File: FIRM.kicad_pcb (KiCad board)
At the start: 4 copper layers, 40.5 x 40.5 mm, 98 parts, among them J2 DM3CS-SF, Q2 IRLML6402, U1 STM32F405RGTx, U2 MIC5219-3.3YM5, U6 A-USBC-20F0-EA-GSR05, U7 W25Q128JVS, X2 32.768khz, Y1 12 MHz

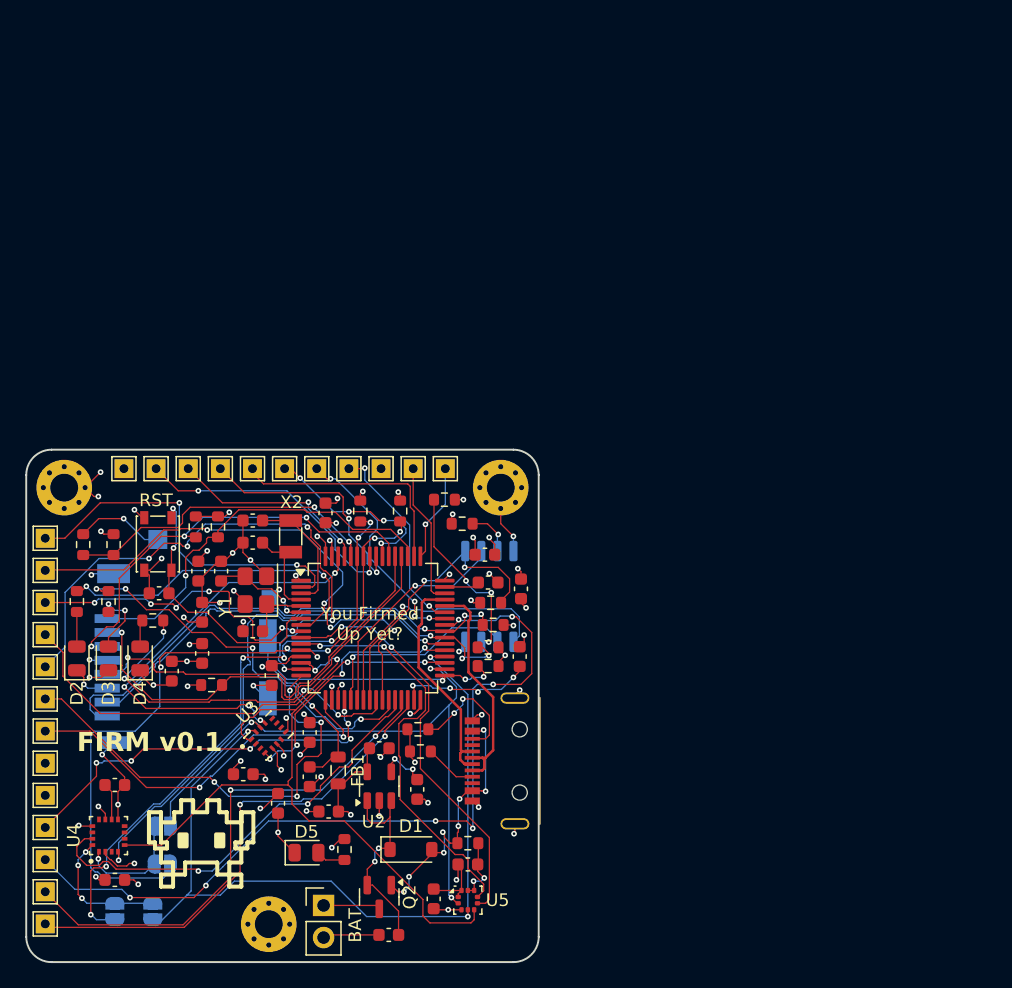
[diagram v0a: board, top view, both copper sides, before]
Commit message: sub 600
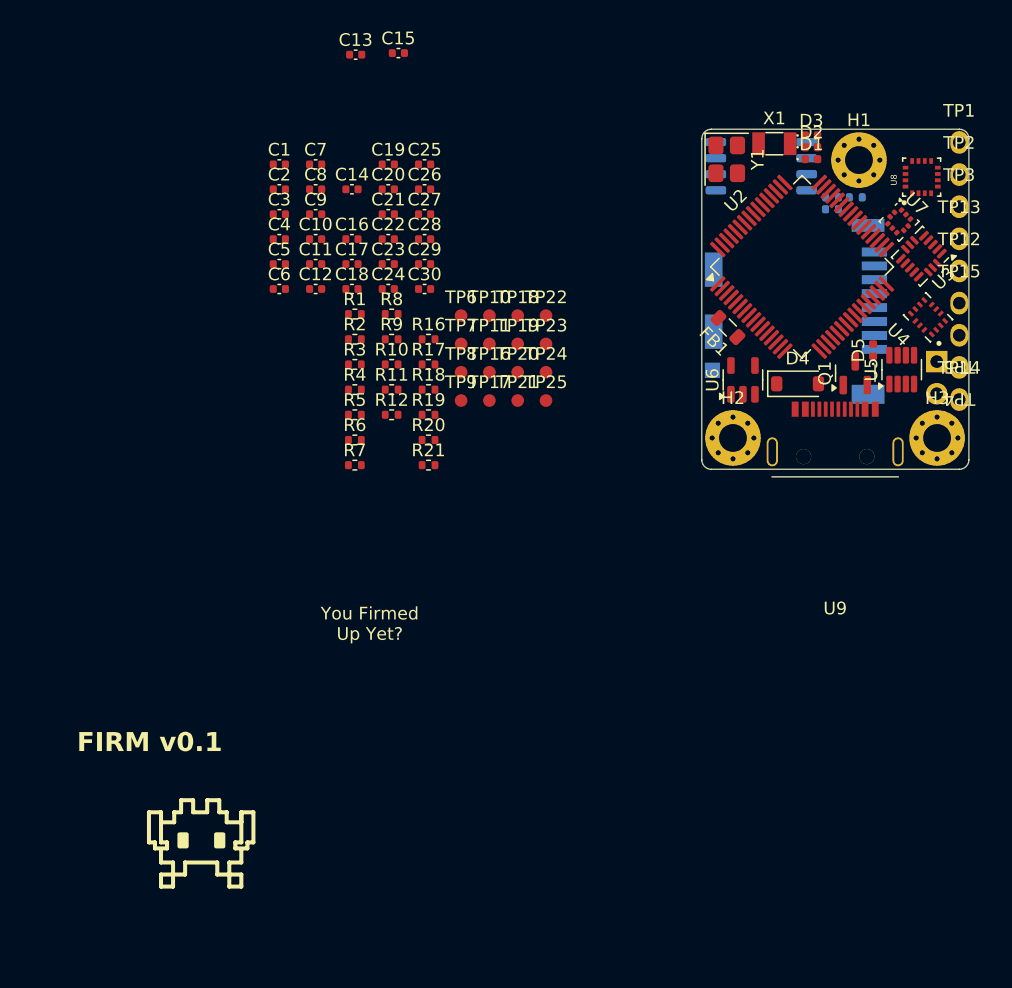
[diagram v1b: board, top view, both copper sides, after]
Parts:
- removed 3.3V: 3.3V Test Point, TestPoint:TestPoint_THTPad_1.5x1.5mm_Drill0.7mm
- removed A0: PA0 Test Point, TestPoint:TestPoint_THTPad_1.5x1.5mm_Drill0.7mm
- removed A1: PA1 Test Point, TestPoint:TestPoint_THTPad_1.5x1.5mm_Drill0.7mm
- removed A10: PA10 Test Point, TestPoint:TestPoint_THTPad_1.5x1.5mm_Drill0.7mm
- removed A15: PA15 Test Point, TestPoint:TestPoint_THTPad_1.5x1.5mm_Drill0.7mm
- removed A2: PA2 Test Point, TestPoint:TestPoint_THTPad_1.5x1.5mm_Drill0.7mm
- removed A3: PA3 Test Point, TestPoint:TestPoint_THTPad_1.5x1.5mm_Drill0.7mm
- removed A4: PA4 Test Point, TestPoint:TestPoint_THTPad_1.5x1.5mm_Drill0.7mm
- removed A8: PA8 Test Point, TestPoint:TestPoint_THTPad_1.5x1.5mm_Drill0.7mm
- removed A9: PA9 Test Point, TestPoint:TestPoint_THTPad_1.5x1.5mm_Drill0.7mm
- removed B10: PB10 Test Point, TestPoint:TestPoint_THTPad_1.5x1.5mm_Drill0.7mm
- removed B11: PB11 Test Point, TestPoint:TestPoint_THTPad_1.5x1.5mm_Drill0.7mm
- removed B3: PB3 Test Point, TestPoint:TestPoint_THTPad_1.5x1.5mm_Drill0.7mm
- removed B4: PB4 Test Point, TestPoint:TestPoint_THTPad_1.5x1.5mm_Drill0.7mm
- removed B5: PB5 Test Point, TestPoint:TestPoint_THTPad_1.5x1.5mm_Drill0.7mm
- removed B8: PB8 Test Point, TestPoint:TestPoint_THTPad_1.5x1.5mm_Drill0.7mm
- removed BAT: Conn_01x02_Pin, Connector_PinHeader_2.54mm:PinHeader_1x02_P2.54mm_Vertical
- removed BOOT0: BOOT0 Pad, TestPoint:TestPoint_Pad_1.5x1.5mm
- removed C0: PC0 Test Point, TestPoint:TestPoint_THTPad_1.5x1.5mm_Drill0.7mm
- removed the C13 at (101.5, 107.0)
- removed the C13 at (117.9, 114.3)
- removed GND (x2): GND Test Point, TestPoint:TestPoint_THTPad_1.5x1.5mm_Drill0.7mm
- removed GND: GND Through-Hole, TestPoint:TestPoint_THTPad_1.5x1.5mm_Drill0.7mm
- removed MOSI: SPI_SDI, Jumper:SolderJumper-2_P1.3mm_Open_RoundedPad1.0x1.5mm
- removed Q2: IRLML6402, Package_TO_SOT_SMD:SOT-23
- removed R22: 5.1k, Resistor_SMD:R_0603_1608Metric
- removed RST: PTS815, Button_Switch_SMD:SW_SPST_PTS810
- removed SCK: SPI_SCK, Jumper:SolderJumper-2_P1.3mm_Open_RoundedPad1.0x1.5mm
- removed SCL: I2C_SCL, Jumper:SolderJumper-2_P1.3mm_Open_RoundedPad1.0x1.5mm
- removed SDA: I2C_SDA, Jumper:SolderJumper-2_P1.3mm_Open_RoundedPad1.0x1.5mm
- removed SWCLK: SWCLK Through-Hole, TestPoint:TestPoint_THTPad_1.5x1.5mm_Drill0.7mm
- removed SWDIO: SWDIO Through-Hole, TestPoint:TestPoint_THTPad_1.5x1.5mm_Drill0.7mm
- removed TP30: PC1 Test Point, TestPoint:TestPoint_THTPad_1.5x1.5mm_Drill0.7mm
- removed X2: 32.768khz, Crystal:Crystal_SMD_3215-2Pin_3.2x1.5mm
- added C13: 100n, Capacitor_SMD:C_0402_1005Metric, F.Cu at (126.0, 68.8)
- added C28: 10u, Capacitor_SMD:C_0402_1005Metric, F.Cu at (131.5, 83.4)
- added C29: 1u, Capacitor_SMD:C_0402_1005Metric, F.Cu at (131.5, 85.3)
- added C30: 10u, Capacitor_SMD:C_0402_1005Metric, F.Cu at (131.5, 87.3)
- added J1: DM3CS-SF, connectors:HRS_DM3CS-SF, B.Cu at (160.7, 88.9)
- added Q1: IRLML6402, Package_TO_SOT_SMD:SOT-23, F.Cu at (165.5, 94.0)
- added R16: 100k, Resistor_SMD:R_0402_1005Metric, F.Cu at (131.8, 91.3)
- added R17: 0.01R, Resistor_SMD:R_0402_1005Metric, F.Cu at (131.8, 93.3)
- added TP1: PA0 Test Point, connectors:Testpoint_1.5x1.5mm_1.0mm, F.Cu at (173.7, 75.7)
- added TP10: I2C1_SCL Test Point, connectors:smd_test_pads_1mm, F.Cu at (136.6, 89.4)
- added TP11: I2C1_SDA Test Point, connectors:smd_test_pads_1mm, F.Cu at (136.6, 91.6)
- added TP12: SWDIO Through-Hole, connectors:Testpoint_1.5x1.5mm_1.0mm, F.Cu at (173.7, 85.9)
- added TP13: SWCLK Through-Hole, connectors:Testpoint_1.5x1.5mm_1.0mm, F.Cu at (173.7, 83.3)
- added TP14: 3.3V Test Point, connectors:Testpoint_1.5x1.5mm_1.0mm, F.Cu at (173.7, 96.0)
- added TP15: GND Test Point, connectors:Testpoint_1.5x1.5mm_1.0mm, F.Cu at (173.7, 88.4)
- added TP16: IMU_CS Test Point, connectors:smd_test_pads_1mm, F.Cu at (136.6, 93.9)
- added TP17: BMP_CS Test Point, connectors:smd_test_pads_1mm, F.Cu at (136.6, 96.1)
- added TP18: MAG_CS Test Point, connectors:smd_test_pads_1mm, F.Cu at (138.8, 89.4)
- added TP19: HIG_CS Test Point, connectors:smd_test_pads_1mm, F.Cu at (138.8, 91.6)
- added TP2: PA1 Test Point, connectors:Testpoint_1.5x1.5mm_1.0mm, F.Cu at (173.7, 78.3)
- added TP20: IMU_INT Test Point, connectors:smd_test_pads_1mm, F.Cu at (138.8, 93.9)
- added TP21: BMP_INT Test Point, connectors:smd_test_pads_1mm, F.Cu at (138.8, 96.1)
- added TP22: MAG_INT Test Point, connectors:smd_test_pads_1mm, F.Cu at (141.1, 89.4)
- added TP23: HIG_INT Test Point, connectors:smd_test_pads_1mm, F.Cu at (141.1, 91.6)
- added TP24: NRST Pad, connectors:smd_test_pads_1mm, F.Cu at (141.1, 93.9)
- added TP25: BOOT0 Pad, connectors:smd_test_pads_1mm, F.Cu at (141.1, 96.1)
- added TP3: PA2 Test Point, connectors:Testpoint_1.5x1.5mm_1.0mm, F.Cu at (173.7, 80.8)
- added TP4: PA9 Test Point, connectors:Testpoint_1.5x1.5mm_1.0mm, F.Cu at (173.7, 93.5)
- added TP5: PA10 Test Point, connectors:Testpoint_1.5x1.5mm_1.0mm, F.Cu at (173.7, 91.0)
- added TP6: PA4 Test Point, connectors:smd_test_pads_1mm, F.Cu at (134.4, 89.4)
- added TP7: MOSI2 Test Point, connectors:smd_test_pads_1mm, F.Cu at (134.4, 91.6)
- added TP8: MISO2 Test Point, connectors:smd_test_pads_1mm, F.Cu at (134.4, 93.9)
- added TP9: SCK2 Test Point, connectors:smd_test_pads_1mm, F.Cu at (134.4, 96.1)
- added U8: ~, sensors:IC_MMC5983MA, F.Cu at (170.8, 78.5)
- added U9: A-USBC-20F0-EA-GSR05, connectors:A-USBC-20F0-EA-GSR05, F.Cu at (163.9, 100.5)
- added X1: 32.768khz, Crystal:Crystal_SMD_3215-2Pin_3.2x1.5mm, F.Cu at (159.1, 75.8)
- C1: value 100n -> 0.1u; footprint Capacitor_SMD:C_0603_1608Metric -> Capacitor_SMD:C_0402_1005Metric
- C10: value 2u2 -> 14p; footprint Capacitor_SMD:C_0603_1608Metric -> Capacitor_SMD:C_0402_1005Metric
- C11, C12: value 6p -> 100n; footprint Capacitor_SMD:C_0603_1608Metric -> Capacitor_SMD:C_0402_1005Metric
- C14: value 14p -> 2u2; footprint Capacitor_SMD:C_0603_1608Metric -> Capacitor_SMD:C_0402_1005Metric
- C15, C8: value 0.1u -> 100n; footprint Capacitor_SMD:C_0603_1608Metric -> Capacitor_SMD:C_0402_1005Metric
- C16: value 1u -> 10n; footprint Capacitor_SMD:C_0603_1608Metric -> Capacitor_SMD:C_0402_1005Metric
- C17: value 10u -> 0.1u; footprint Capacitor_SMD:C_0603_1608Metric -> Capacitor_SMD:C_0402_1005Metric
- C18, C19, C20, C21, C24, C25, C27, C3, C9: footprint Capacitor_SMD:C_0603_1608Metric -> Capacitor_SMD:C_0402_1005Metric
- C2: value 100n -> 4u7; footprint Capacitor_SMD:C_0603_1608Metric -> Capacitor_SMD:C_0402_1005Metric
- C22: value 10u -> 100n; footprint Capacitor_SMD:C_0603_1608Metric -> Capacitor_SMD:C_0402_1005Metric
- C23: value 470p -> 100n; footprint Capacitor_SMD:C_0603_1608Metric -> Capacitor_SMD:C_0402_1005Metric
- C26: value 100n -> 470p; footprint Capacitor_SMD:C_0603_1608Metric -> Capacitor_SMD:C_0402_1005Metric
- C4: value 100n -> 6p; footprint Capacitor_SMD:C_0603_1608Metric -> Capacitor_SMD:C_0402_1005Metric
- C5: value 100n -> 14p; footprint Capacitor_SMD:C_0603_1608Metric -> Capacitor_SMD:C_0402_1005Metric
- C6: value 4u7 -> 100n; footprint Capacitor_SMD:C_0603_1608Metric -> Capacitor_SMD:C_0402_1005Metric
- C7: value 10n -> 6p; footprint Capacitor_SMD:C_0603_1608Metric -> Capacitor_SMD:C_0402_1005Metric
- D1: value D_Schottky -> LED_Blue; footprint Diode_SMD:D_SOD-123 -> LED_SMD:LED_0402_1005Metric
- D2: value LED -> LED_Yellow; footprint LED_SMD:LED_0805_2012Metric -> LED_SMD:LED_0402_1005Metric
- D3: value LED -> LED_Red; footprint LED_SMD:LED_0805_2012Metric -> LED_SMD:LED_0402_1005Metric
- D4: value LED -> D_Schottky; footprint LED_SMD:LED_0805_2012Metric -> Diode_SMD:D_SOD-123
- D5: value LED -> LED_Green; footprint LED_SMD:LED_0805_2012Metric -> LED_SMD:LED_0402_1005Metric
- J2: value DM3CS-SF -> Conn_01x02_Pin; footprint DM3CS-SF:HRS_DM3CS-SF -> connectors:power_headers; moved to F.Cu
- R1: value 100k -> 10k; footprint Resistor_SMD:R_0603_1608Metric -> Resistor_SMD:R_0402_1005Metric
- R10: value 330 -> 47k; footprint Resistor_SMD:R_0603_1608Metric -> Resistor_SMD:R_0402_1005Metric
- R11: value 1k2 -> 3k3; footprint Resistor_SMD:R_0603_1608Metric -> Resistor_SMD:R_0402_1005Metric
- R12: value 1k5 -> 3k3; footprint Resistor_SMD:R_0603_1608Metric -> Resistor_SMD:R_0402_1005Metric
- R13: value 10k -> 330; footprint Resistor_SMD:R_0603_1608Metric -> Resistor_SMD:R_0402_1005Metric; moved to B.Cu
- R14: value 10k -> 1k2; footprint Resistor_SMD:R_0603_1608Metric -> Resistor_SMD:R_0402_1005Metric; moved to B.Cu
- R15: value 1k2 -> 1k5; footprint Resistor_SMD:R_0603_1608Metric -> Resistor_SMD:R_0402_1005Metric; moved to B.Cu
- R18: value 2k2 -> 1k2; footprint Resistor_SMD:R_0603_1608Metric -> Resistor_SMD:R_0402_1005Metric
- R19: value 2k2 -> 100; footprint Resistor_SMD:R_0603_1608Metric -> Resistor_SMD:R_0402_1005Metric
- R2, R4, R7: footprint Resistor_SMD:R_0603_1608Metric -> Resistor_SMD:R_0402_1005Metric
- R20: value 100 -> 5.1k; footprint Resistor_SMD:R_0603_1608Metric -> Resistor_SMD:R_0402_1005Metric
- R21: value 10k -> 5.1k; footprint Resistor_SMD:R_0603_1608Metric -> Resistor_SMD:R_0402_1005Metric
- R3: value 47k -> 100k; footprint Resistor_SMD:R_0603_1608Metric -> Resistor_SMD:R_0402_1005Metric
- R5, R6: value 47k -> 10k; footprint Resistor_SMD:R_0603_1608Metric -> Resistor_SMD:R_0402_1005Metric
- R8: value 100k -> 47k; footprint Resistor_SMD:R_0603_1608Metric -> Resistor_SMD:R_0402_1005Metric
- R9: value 5.1k -> 47k; footprint Resistor_SMD:R_0603_1608Metric -> Resistor_SMD:R_0402_1005Metric
- U1: value STM32F405RGTx -> W25Q128JVS; footprint Package_QFP:LQFP-64_10x10mm_P0.5mm -> Package_SO:SOIC-8_5.3x5.3mm_P1.27mm; moved to B.Cu
- U2: value MIC5219-3.3YM5 -> STM32F405RGTx; footprint Package_TO_SOT_SMD:SOT-23-5 -> Package_QFP:LQFP-64_10x10mm_P0.5mm
- U3: value ~ -> ADXL371; footprint sensors:IC_ICM-45686 -> Sensor_Motion:Analog_LGA-16_3.25x3mm_P0.5mm_LayoutBorder3x5y
- U4: footprint sensors:IC_MMC5983MA -> sensors:IC_ICM-45686
- U5: value ~ -> INA219AxDCN; footprint Package_LGA:ST_HLGA-10_2x2mm_P0.5mm_LayoutBorder3x2y -> Package_TO_SOT_SMD:SOT-23-8
- U6: value A-USBC-20F0-EA-GSR05 -> MIC5219-3.3YM5; footprint connectors:A-USBC-20F0-EA-GSR05 -> Package_TO_SOT_SMD:SOT-23-5
- U7: value W25Q128JVS -> ~; footprint Package_SO:SOIC-8_5.3x5.3mm_P1.27mm -> sensors:BMPFootprintNoSolderMask; moved to F.Cu
- moved U4 76.6 mm to (171.3, 89.5), turned to 135 degrees
- moved H1 76.3 mm to (165.8, 77.1)
- moved D2 70.7 mm to (162.1, 76.1), turned to 0 degrees
- moved D3 69.2 mm to (162.0, 75.2), turned to 0 degrees
- moved H3 69.1 mm to (172.0, 99.1)
- moved R15 65.5 mm to (165.6, 80.1), turned to 0 degrees
- moved U3 64.0 mm to (170.7, 84.7), turned to -135 degrees
- moved J2 63.7 mm to (172.0, 93.0), turned to 0 degrees
- moved D1 63.1 mm to (162.1, 77.0)
- moved D5 59.9 mm to (166.9, 92.1), turned to 90 degrees
- moved C19 58.2 mm to (128.6, 77.5), turned to 0 degrees
- moved D4 56.3 mm to (161.0, 94.8), turned to 0 degrees
- moved C22 55.0 mm to (128.6, 83.4), turned to 0 degrees
- moved U5 54.2 mm to (169.2, 93.7), turned to 90 degrees
- moved C26 53.5 mm to (131.5, 79.4), turned to 0 degrees
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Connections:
- C1 pad 1: +3.3V -> /NRST
- C10 pad 1: /VCAP2 -> /HSE_OUT
- C11 pad 1: /LSE_IN -> GND
- C11 pad 2: GND -> +3.3V
- C12 pad 1: /LSE_OUT -> GND
- C12 pad 2: GND -> +3.3V
- C14 pad 1: /HSE_OUT -> /VCAP2
- C15 pad 1: /NRST -> +3.3V
- C16 pad 1: +3.3V -> Net-(U2-VDDA)
- C17 pad 1: GND -> Net-(U2-VDDA)
- C17 pad 2: Net-(U4-CAP) -> GND
- C19 pad 1: +3.3V -> GND
- C19 pad 2: GND -> +3.3V
- C20 pad 1: +3.3V -> GND
- C20 pad 2: GND -> +3.3V
- C21 pad 1: GND -> +3.3V
- C21 pad 2: +3.3V -> GND
- C22 pad 1: Net-(D1-K) -> +3.3V
- C23 pad 1: Net-(U2-BP) -> GND
- C23 pad 2: GND -> +3.3V
- C24 pad 1: +3.3V -> /VSENS_OUT
- C26 pad 1: GND -> Net-(U6-BP)
- C26 pad 2: +3.3V -> GND
- C4 pad 1: +3.3V -> /LSE_IN
- C5 pad 1: +3.3V -> /HSE_IN
- C7 pad 1: Net-(U1-VDDA) -> /LSE_OUT
- C8 pad 1: Net-(U1-VDDA) -> +3.3V
- D1 pad 1: Net-(D1-K) -> GND
- D1 pad 2: VBUS -> Net-(D1-A)
- D4 pad 1: GND -> /VSENS_IN
- D4 pad 2: Net-(D4-A) -> VBUS
- FB1 pad 1: Net-(U1-VDDA) -> Net-(U2-VDDA)
- J2 pad 1: /SDIO_D2 -> VBAT
- J2 pad 2: /SDIO_D3 -> GND
- R1 pad 1: /BOOT0 -> +3.3V
- R1 pad 2: GND -> Net-(U1-~{HOLD}/~{RESET}/IO_{3})
- R10 pad 1: Net-(D2-A) -> /SDIO_D2
- R10 pad 2: /DBUG_0 -> +3.3V
- R11 pad 1: Net-(D3-A) -> /I2C1_SCL
- R11 pad 2: /DBUG_1 -> +3.3V
- R12 pad 1: Net-(D4-A) -> /I2C1_SDA
- R12 pad 2: /DBUG_2 -> +3.3V
- R13 pad 1: +3.3V -> Net-(D1-A)
- R13 pad 2: Net-(U7-~{HOLD}/~{RESET}/IO_{3}) -> /DBUG_0
- R14 pad 1: +3.3V -> Net-(D2-A)
- R14 pad 2: Net-(U7-~{WP}/IO_{2}) -> /DBUG_1
- R15 pad 1: Net-(D5-A) -> Net-(D3-A)
- R15 pad 2: +3.3V -> /DBUG_2
- R18 pad 1: /I2C1_SCL -> Net-(D5-A)
- R19 pad 1: /I2C1_SDA -> Net-(R19-Pad1)
- R19 pad 2: +3.3V -> /BOOT0
- R2 pad 1: /SDIO_D2 -> /SDIO_D1
- R20 pad 2: /BOOT0 -> GND
- R21 pad 1: +3.3V -> Net-(U9-CC2)
- R21 pad 2: /FLASH_CS -> GND
- R3 pad 1: /SDIO_D3 -> /BOOT0
- R3 pad 2: +3.3V -> GND
- R4 pad 1: /SDIO_CMD -> /SDIO_D0
- R5 pad 1: /SDIO_D0 -> +3.3V
- R5 pad 2: +3.3V -> Net-(U1-~{WP}/IO_{2})
- R6 pad 1: /SDIO_D1 -> +3.3V
- R6 pad 2: +3.3V -> /SD_DETECT
- R7 pad 2: /SD_DETECT -> /FLASH_CS
- R8 pad 1: VBUS -> /SDIO_CMD
- R8 pad 2: GND -> +3.3V
- R9 pad 1: Net-(U6-CC1) -> /SDIO_D3
- R9 pad 2: GND -> +3.3V
- U1 pad 1: +3.3V -> /FLASH_CS
- U1 pad 2: /PC13 -> /MISO1
- U1 pad 3: /LSE_IN -> Net-(U1-~{WP}/IO_{2})
- U1 pad 4: /LSE_OUT -> GND
- U1 pad 5: /HSE_IN -> /MOSI1
- U1 pad 6: /HSE_OUT -> /SCK1
- U1 pad 7: /NRST -> Net-(U1-~{HOLD}/~{RESET}/IO_{3})
- U1 pad 8: /PC0 -> +3.3V
- U2 pad 1: Net-(D1-K) -> +3.3V
- U2 pad 2: GND -> /PC13
- U2 pad 3: Net-(D1-K) -> /LSE_IN
- U2 pad 4: Net-(U2-BP) -> /LSE_OUT
- U2 pad 5: +3.3V -> /HSE_IN
- U3 pad 1: /MISO2 -> +3.3V
- U3 pad 11: unconnected-(U3-RESV/AUX1_SDO-Pad11) -> /HIG_INT
- U3 pad 12: /IMU_CS -> GND
- U3 pad 13: /SCK2 -> GND
- U3 pad 14: /MOSI2 -> +3.3V
- U3 pad 4: /IMU_INT -> /SCK2
- U3 pad 5: +3.3V -> unconnected-(U3-RES-Pad5)
- U3 pad 6: GND -> /MOSI2
- U3 pad 7: unconnected-(U3-RESV-Pad7) -> /MISO2
- U3 pad 8: +3.3V -> /HIG_CS
- U4 pad 1: Net-(JP3-A) -> /MISO2
- U4 pad 10: Net-(U4-CAP) -> unconnected-(U4-RESV/AUX1_CS-Pad10)
- U4 pad 11: GND -> unconnected-(U4-RESV/AUX1_SDO-Pad11)
- U4 pad 12: unconnected-(U4-NC-Pad12) -> /IMU_CS
- U4 pad 13: +3.3V -> /SCK2
- U4 pad 14: unconnected-(U4-NC-Pad14) -> /MOSI2
- U4 pad 2: +3.3V -> unconnected-(U4-RESV/AUX1_SDIO/AUX1_SDI/MAS_DA-Pad2)
- U4 pad 4: /MAG_CS -> /IMU_INT
- U4 pad 5: /MISO2 -> +3.3V
- U4 pad 6: unconnected-(U4-NC-Pad6) -> GND
- U4 pad 8: unconnected-(U4-NC-Pad8) -> +3.3V
- U4 pad 9: GND -> unconnected-(U4-INT2/FSYNC/CLKIN-Pad9)
- U5 pad 1: +3.3V -> /VSENS_IN
- U5 pad 2: /SCK2 -> /VSENS_OUT
- U5 pad 4: /MOSI2 -> +3.3V
- U5 pad 5: /MISO2 -> /I2C1_SCL
- U5 pad 6: /BMP_CS -> /I2C1_SDA
- U5 pad 7: /BMP_INT -> GND
- U7 pad 1: /FLASH_CS -> +3.3V
- U7 pad 2: /MISO1 -> /SCK2
- U7 pad 3: Net-(U7-~{WP}/IO_{2}) -> GND
- U7 pad 4: GND -> /MOSI2
- U7 pad 5: /MOSI1 -> /MISO2
- U7 pad 6: /SCK1 -> /BMP_CS
- U7 pad 7: Net-(U7-~{HOLD}/~{RESET}/IO_{3}) -> /BMP_INT
- U7 pad 8: +3.3V -> GND
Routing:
- net GND: track 94.7 -> 0.00 mm, vias 47 -> 0
- net /MOSI2: track 66.4 -> 0.00 mm, vias 3 -> 0
- net /PA8: track 65.2 -> 0.00 mm, vias 7 -> 0
- net /MISO2: track 62.5 -> 0.00 mm, vias 2 -> 0
- net +3.3V: track 56.0 -> 0.00 mm, vias 33 -> 0
- net /I2C1_SCL: track 55.9 -> 0.00 mm, vias 5 -> 0
- net /SCK2: track 50.0 -> 0.00 mm, vias 3 -> 0
- net /I2C1_SDA: track 47.7 -> 0.00 mm, vias 7 -> 0
- net /PA1: track 45.6 -> 0.00 mm, vias 5 -> 0
- net /MAG_CS: track 41.4 -> 0.00 mm, vias 2 -> 0
- net /PB10: track 41.1 -> 0.00 mm, vias 2 -> 0
- net /PB11: track 39.9 -> 0.00 mm, vias 2 -> 0
- net /SDIO_D1: track 39.6 -> 0.00 mm, vias 3 -> 0
- net /SDIO_D0: track 37.7 -> 0.00 mm, vias 3 -> 0
- net /DBUG_0: track 37.3 -> 0.00 mm, vias 4 -> 0
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- removed copper zone on In2.Cu, net +3.3V
- removed copper zone on In1.Cu, net GND
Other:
- board size 40.5 x 40.5 mm -> 21.1 x 26.9 mm
